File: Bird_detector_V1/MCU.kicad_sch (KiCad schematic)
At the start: 2 parts, among them U1 ESP32-S3-MINI-1, U2 ESP32-S3-WROOM-1

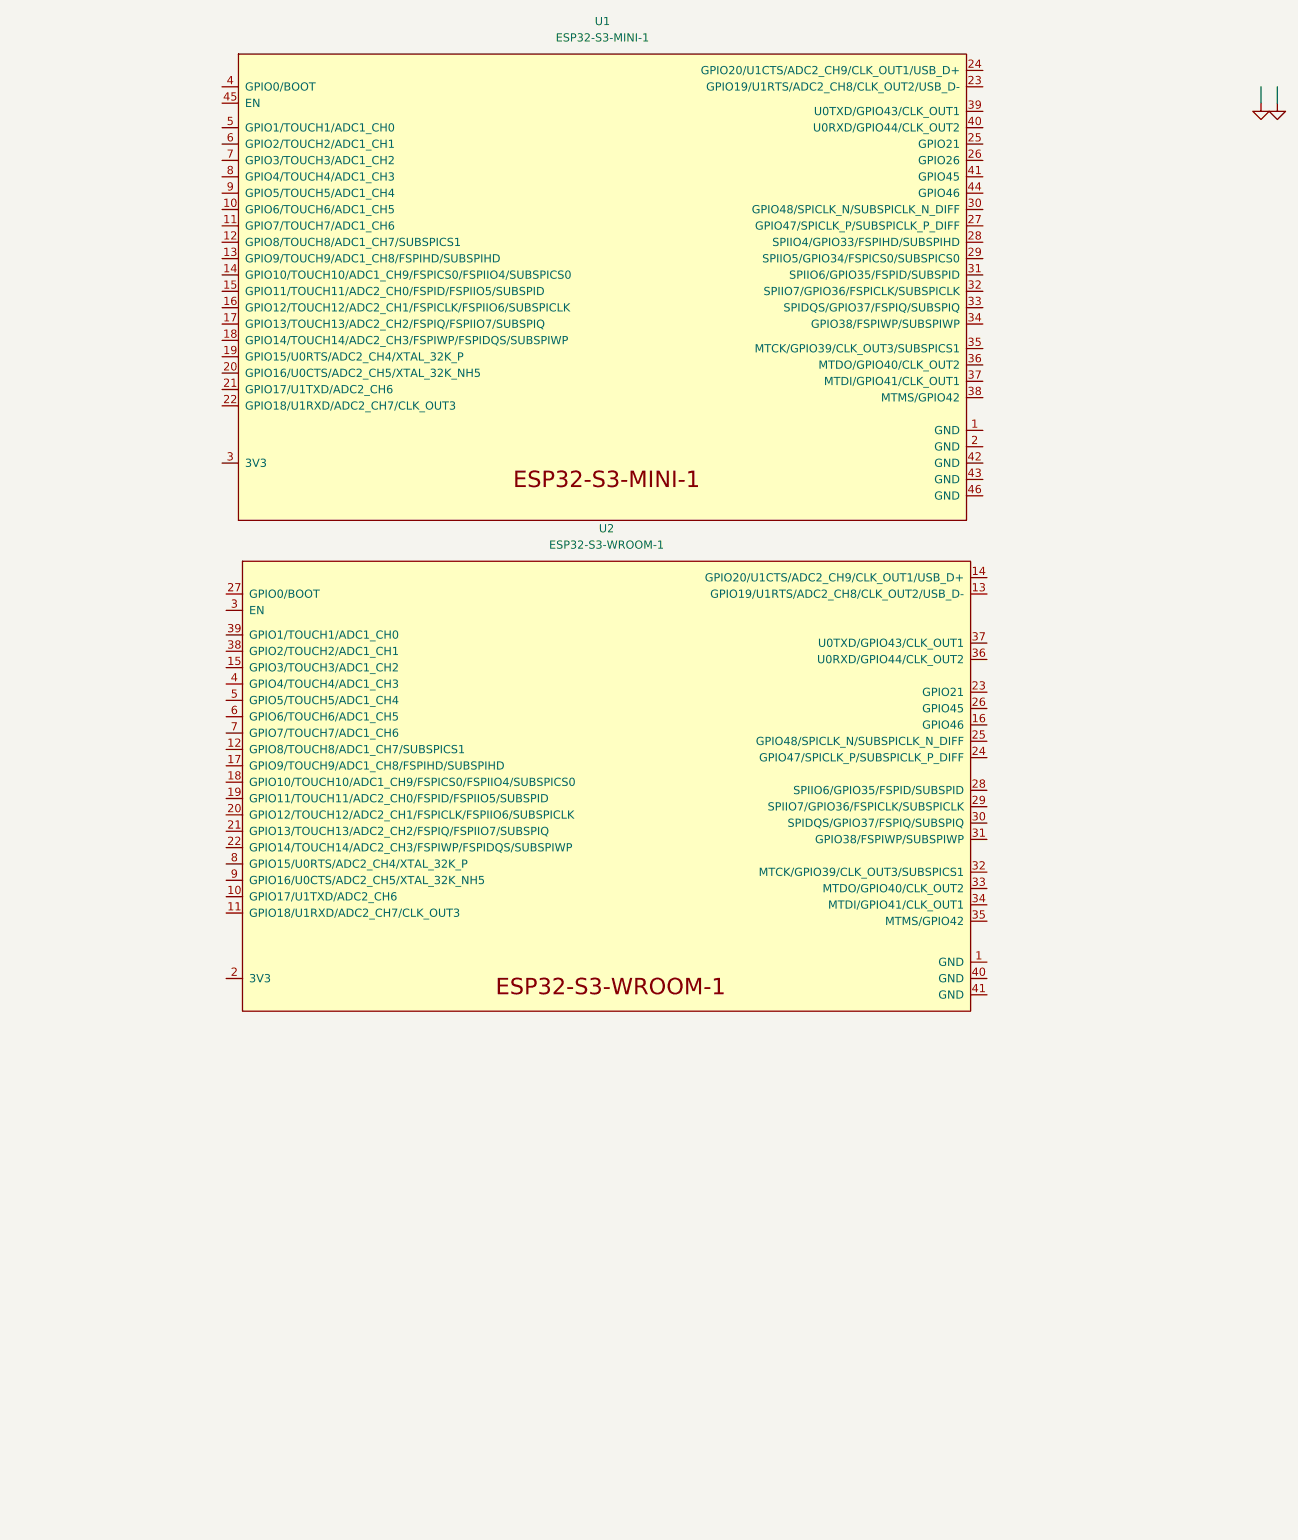
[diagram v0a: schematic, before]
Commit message: g
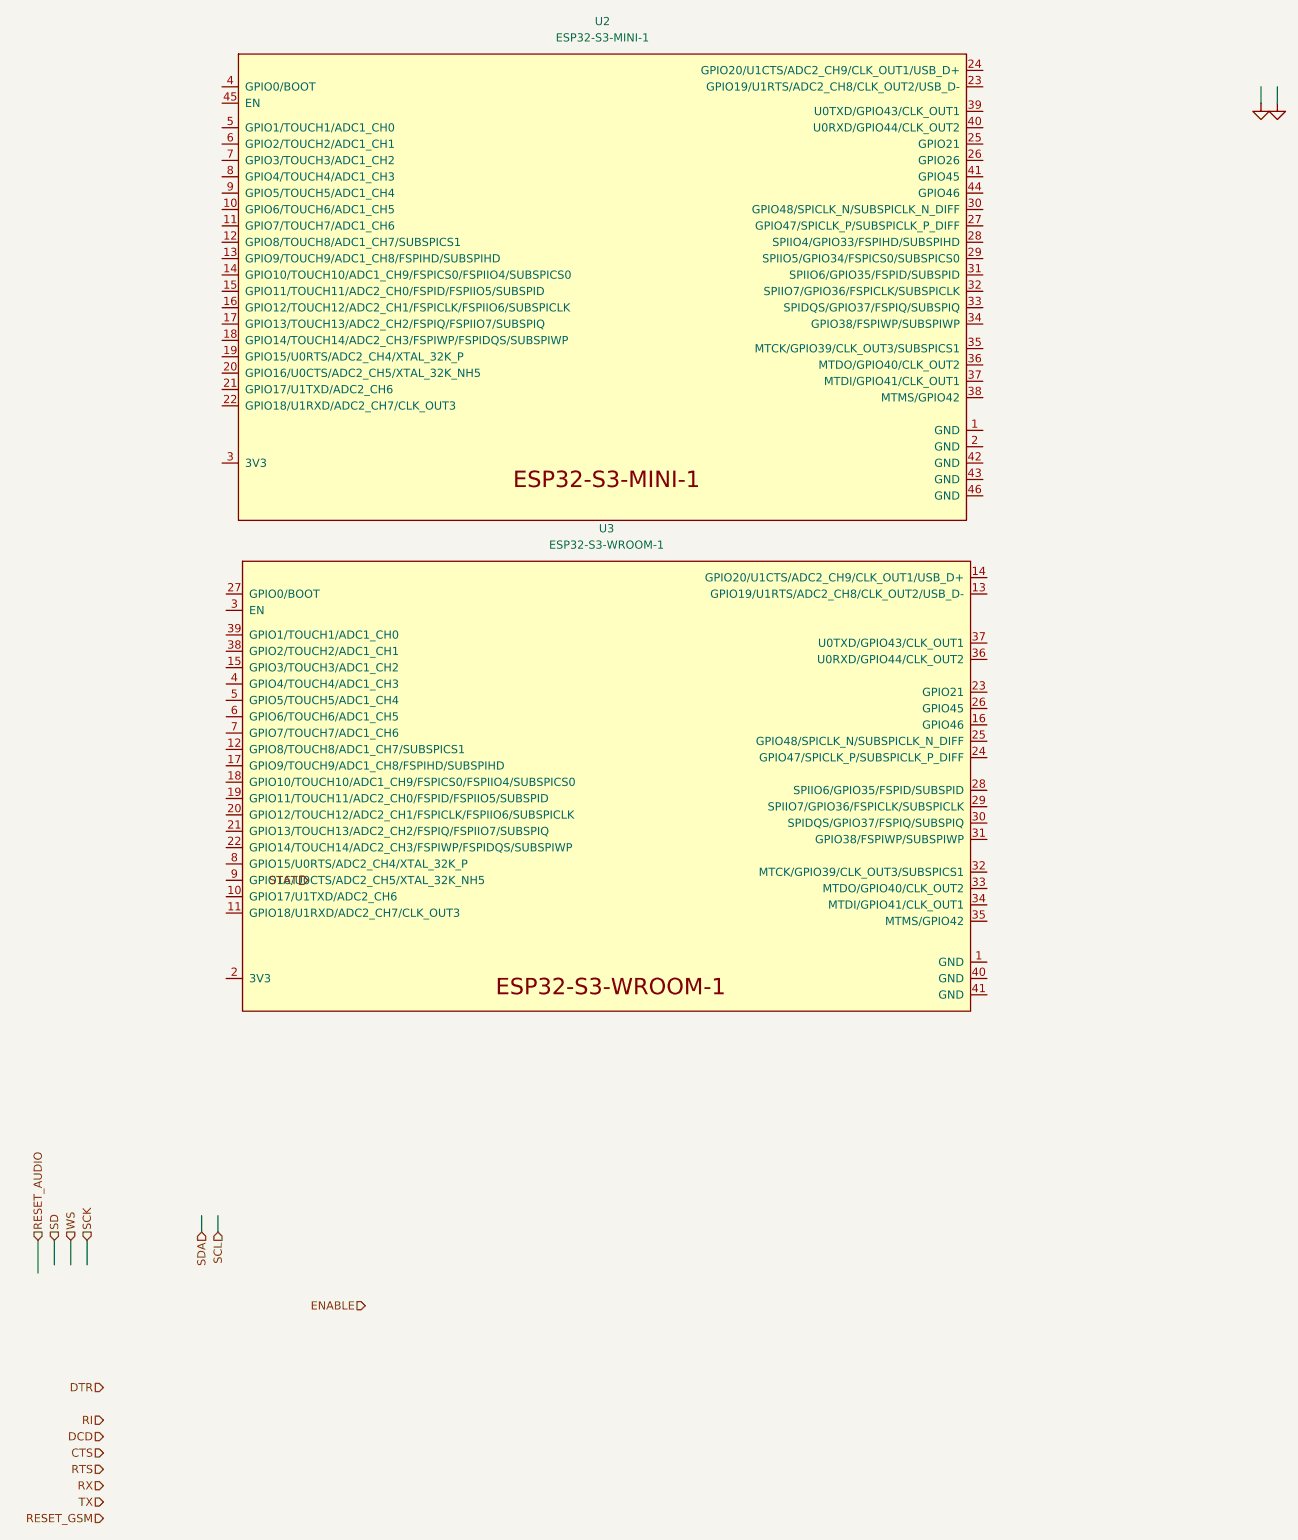
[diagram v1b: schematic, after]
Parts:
- renumbered U1 to U2, U2 to U3
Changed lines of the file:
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@@
 (kicad_sch (version 20211123) (generator eeschema)
   (paper "A3")
+  (wire (pts (xy 31.75 233.68) (xy 31.75 237.49))
+    (stroke (width 0) (type default) (color 0 0 0 0))
+  )
+  (wire (pts (xy 29.21 238.76) (xy 29.21 233.68))
+    (stroke (width 0) (type default) (color 0 0 0 0))
+  )
   (wire (pts (xy 221.615 54.61) (xy 221.615 57.15))
     (stroke (width 0) (type default) (color 0 0 0 0))
   )
+  (wire (pts (xy 36.83 233.68) (xy 36.83 237.49))
+    (stroke (width 0) (type default) (color 0 0 0 0))
+  )
+  (wire (pts (xy 34.29 233.68) (xy 34.29 237.49))
+    (stroke (width 0) (type default) (color 0 0 0 0))
+  )
+  (wire (pts (xy 54.61 229.87) (xy 54.61 232.41))
+    (stroke (width 0) (type default) (color 0 0 0 0))
+  )
   (wire (pts (xy 219.075 54.61) (xy 219.075 57.15))
     (stroke (width 0) (type default) (color 0 0 0 0))
   )
+  (wire (pts (xy 57.15 229.87) (xy 57.15 232.41))
+    (stroke (width 0) (type default) (color 0 0 0 0))
+  )
+  (hierarchical_label "DTR" (shape input) (at 39.37 256.54 180)
+    (effects (font (size 1.27 1.27)) (justify right))
+  )
+  (hierarchical_label "SCK" (shape input) (at 36.83 233.68 90)
+    (effects (font (size 1.27 1.27)) (justify left))
+  )
+  (hierarchical_label "STAT" (shape input) (at 71.12 177.8 180)
+    (effects (font (size 1.27 1.27)) (justify right))
+  )
+  (hierarchical_label "CTS" (shape input) (at 39.37 266.7 180)
+    (effects (font (size 1.27 1.27)) (justify right))
+  )
+  (hierarchical_label "SD" (shape input) (at 31.75 233.68 90)
+    (effects (font (size 1.27 1.27)) (justify left))
+  )
+  (hierarchical_label "RX" (shape input) (at 39.37 271.78 180)
+    (effects (font (size 1.27 1.27)) (justify right))
+  )
+  (hierarchical_label "RTS" (shape input) (at 39.37 269.24 180)
+    (effects (font (size 1.27 1.27)) (justify right))
+  )
+  (hierarchical_label "SDA" (shape input) (at 54.61 232.41 270)
+    (effects (font (size 1.27 1.27)) (justify right))
+  )
+  (hierarchical_label "DCD" (shape input) (at 39.37 264.16 180)
+    (effects (font (size 1.27 1.27)) (justify right))
+  )
+  (hierarchical_label "RI" (shape input) (at 39.37 261.62 180)
+    (effects (font (size 1.27 1.27)) (justify right))
+  )
+  (hierarchical_label "RESET_AUDIO" (shape input) (at 29.21 233.68 90)
+    (effects (font (size 1.27 1.27)) (justify left))
+  )
+  (hierarchical_label "RESET_GSM" (shape input) (at 39.37 276.86 180)
+    (effects (font (size 1.27 1.27)) (justify right))
+  )
+  (hierarchical_label "ENABLE" (shape input) (at 80.01 243.84 180)
+    (effects (font (size 1.27 1.27)) (justify right))
+  )
+  (hierarchical_label "TX" (shape input) (at 39.37 274.32 180)
+    (effects (font (size 1.27 1.27)) (justify right))
+  )
+  (hierarchical_label "WS" (shape input) (at 34.29 233.68 90)
+    (effects (font (size 1.27 1.27)) (justify left))
+  )
+  (hierarchical_label "SCL" (shape input) (at 57.15 232.41 270)
+    (effects (font (size 1.27 1.27)) (justify right))
+  )
   (symbol (lib_id "Espressif:ESP32-S3-MINI-1") (at 117.475 83.82 0) (unit 1)
     (in_bom yes) (on_board yes) (fields_autoplaced)
-    (property "Reference" "U1" (id 0) (at 116.84 44.45 0))
+    (property "Reference" "U2" (id 0) (at 116.84 44.45 0))
     (property "Value" "ESP32-S3-MINI-1" (id 1) (at 116.84 46.99 0))
     (property "Footprint" "Espressif:ESP32-S3-MINI-1" (id 2) (at 117.475 125.73 0)
@@
   (symbol (lib_id "Espressif:ESP32-S3-WROOM-1") (at 118.11 162.56 0) (unit 1)
     (in_bom yes) (on_board yes) (fields_autoplaced)
-    (property "Reference" "U2" (id 0) (at 117.475 123.19 0))
+    (property "Reference" "U3" (id 0) (at 117.475 123.19 0))
     (property "Value" "ESP32-S3-WROOM-1" (id 1) (at 117.475 125.73 0))
     (property "Footprint" "Espressif:ESP32-S3-WROOM-1" (id 2) (at 118.11 201.93 0)
@@
   (symbol (lib_id "power:GND") (at 221.615 57.15 0) (unit 1)
     (in_bom yes) (on_board yes) (fields_autoplaced)
-    (property "Reference" "#PWR020" (id 0) (at 221.615 63.5 0)
+    (property "Reference" "#PWR036" (id 0) (at 221.615 63.5 0)
       (effects (font (size 1.27 1.27)) hide)
     )
@@
   (symbol (lib_id "power:GND") (at 219.075 57.15 0) (unit 1)
     (in_bom yes) (on_board yes) (fields_autoplaced)
-    (property "Reference" "#PWR019" (id 0) (at 219.075 63.5 0)
-      (effects (font (size 1.27 1.27)) hide)
-    )
+    (property "Reference" "#PWR035" (id 0) (at 219.075 63.5 0)
+      (effects (font (size 1.27 1.27)) hide)
+    )
